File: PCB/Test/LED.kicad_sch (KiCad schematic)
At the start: 45 parts

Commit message: Tidy
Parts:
- TP1, TP2, TP3, TP4, TP5: now left out of the parts list
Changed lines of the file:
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@@
 		(unit 1)
 		(exclude_from_sim no)
-		(in_bom yes)
+		(in_bom no)
 		(on_board yes)
 		(dnp no)
@@
 		(unit 1)
 		(exclude_from_sim no)
-		(in_bom yes)
+		(in_bom no)
 		(on_board yes)
 		(dnp no)
@@
 		(unit 1)
 		(exclude_from_sim no)
-		(in_bom yes)
+		(in_bom no)
 		(on_board yes)
 		(dnp no)
@@
 		(unit 1)
 		(exclude_from_sim no)
-		(in_bom yes)
+		(in_bom no)
 		(on_board yes)
 		(dnp no)
@@
 		(unit 1)
 		(exclude_from_sim no)
-		(in_bom yes)
-		(on_board yes)
-		(dnp no)
+		(in_bom no)
+		(on_board yes)
+		(dnp no)

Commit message: Tweaked design
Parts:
- D11, D12, D13, D14, D15, D16, D17, D18, D19, D20: value XL-1010RGBC-WS2812B -> XL-1615RGBC-WS2812B
- D21, D22, D23, D24, D25, D26, D27, D28, D29, D30, D31, D32, D33, D34, D35, D36, D37, D38, D39, D40: value XL-1010RGBC-WS2812B -> XL-2020RGBC-WS2812B
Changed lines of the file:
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@@
 			)
 		)
-		(property "Value" "XL-1010RGBC-WS2812B"
+		(property "Value" "XL-1615RGBC-WS2812B"
 			(at 160.02 99.06 0)
 			(effects
@@
 			)
 		)
-		(property "Value" "XL-1010RGBC-WS2812B"
+		(property "Value" "XL-2020RGBC-WS2812B"
 			(at 113.665 139.065 0)
 			(effects
@@
 			)
 		)
-		(property "Value" "XL-1010RGBC-WS2812B"
+		(property "Value" "XL-1615RGBC-WS2812B"
 			(at 137.16 99.06 0)
 			(effects
@@
 			)
 		)
-		(property "Value" "XL-1010RGBC-WS2812B"
+		(property "Value" "XL-2020RGBC-WS2812B"
 			(at 174.625 139.065 0)
 			(effects
@@
 			)
 		)
-		(property "Value" "XL-1010RGBC-WS2812B"
+		(property "Value" "XL-1615RGBC-WS2812B"
 			(at 144.78 99.06 0)
 			(effects
@@
 			)
 		)
-		(property "Value" "XL-1010RGBC-WS2812B"
+		(property "Value" "XL-2020RGBC-WS2812B"
 			(at 113.665 119.38 0)
 			(effects
@@
 			)
 		)
-		(property "Value" "XL-1010RGBC-WS2812B"
+		(property "Value" "XL-1615RGBC-WS2812B"
 			(at 121.92 99.06 0)
 			(effects
@@
 			)
 		)
-		(property "Value" "XL-1010RGBC-WS2812B"
+		(property "Value" "XL-1615RGBC-WS2812B"
 			(at 175.26 99.06 0)
 			(effects
@@
 			)
 		)
-		(property "Value" "XL-1010RGBC-WS2812B"
+		(property "Value" "XL-2020RGBC-WS2812B"
 			(at 159.385 119.38 0)
 			(effects
@@
 			)
 		)
-		(property "Value" "XL-1010RGBC-WS2812B"
+		(property "Value" "XL-2020RGBC-WS2812B"
 			(at 144.145 139.065 0)
 			(effects
@@
 			)
 		)
-		(property "Value" "XL-1010RGBC-WS2812B"
+		(property "Value" "XL-2020RGBC-WS2812B"
 			(at 106.045 139.065 0)
 			(effects
@@
 			)
 		)
-		(property "Value" "XL-1010RGBC-WS2812B"
+		(property "Value" "XL-2020RGBC-WS2812B"
 			(at 144.145 119.38 0)
 			(effects
@@
 			)
 		)
-		(property "Value" "XL-1010RGBC-WS2812B"
+		(property "Value" "XL-2020RGBC-WS2812B"
 			(at 106.045 119.38 0)
 			(effects
@@
 			)
 		)
-		(property "Value" "XL-1010RGBC-WS2812B"
+		(property "Value" "XL-2020RGBC-WS2812B"
 			(at 136.525 139.065 0)
 			(effects
@@
 			)
 		)
-		(property "Value" "XL-1010RGBC-WS2812B"
+		(property "Value" "XL-2020RGBC-WS2812B"
 			(at 151.765 119.38 0)
 			(effects
@@
 			)
 		)
-		(property "Value" "XL-1010RGBC-WS2812B"
+		(property "Value" "XL-1615RGBC-WS2812B"
 			(at 152.4 99.06 0)
 			(effects
@@
 			)
 		)
-		(property "Value" "XL-1010RGBC-WS2812B"
+		(property "Value" "XL-2020RGBC-WS2812B"
 			(at 121.285 119.38 0)
 			(effects
@@
 			)
 		)
-		(property "Value" "XL-1010RGBC-WS2812B"
+		(property "Value" "XL-2020RGBC-WS2812B"
 			(at 174.625 119.38 0)
 			(effects
@@
 			)
 		)
-		(property "Value" "XL-1010RGBC-WS2812B"
+		(property "Value" "XL-2020RGBC-WS2812B"
 			(at 159.385 139.065 0)
 			(effects
@@
 			)
 		)
-		(property "Value" "XL-1010RGBC-WS2812B"
+		(property "Value" "XL-1615RGBC-WS2812B"
 			(at 129.54 99.06 0)
 			(effects
@@
 			)
 		)
-		(property "Value" "XL-1010RGBC-WS2812B"
+		(property "Value" "XL-1615RGBC-WS2812B"
 			(at 167.64 99.06 0)
 			(effects
@@
 			)
 		)
-		(property "Value" "XL-1010RGBC-WS2812B"
+		(property "Value" "XL-2020RGBC-WS2812B"
 			(at 167.005 119.38 0)
 			(effects
@@
 			)
 		)
-		(property "Value" "XL-1010RGBC-WS2812B"
+		(property "Value" "XL-2020RGBC-WS2812B"
 			(at 121.285 139.065 0)
 			(effects
@@
 			)
 		)
-		(property "Value" "XL-1010RGBC-WS2812B"
+		(property "Value" "XL-2020RGBC-WS2812B"
 			(at 167.005 139.065 0)
 			(effects
@@
 			)
 		)
-		(property "Value" "XL-1010RGBC-WS2812B"
+		(property "Value" "XL-2020RGBC-WS2812B"
 			(at 128.905 119.38 0)
 			(effects
@@
 			)
 		)
-		(property "Value" "XL-1010RGBC-WS2812B"
+		(property "Value" "XL-2020RGBC-WS2812B"
 			(at 151.765 139.065 0)
 			(effects
@@
 			)
 		)
-		(property "Value" "XL-1010RGBC-WS2812B"
+		(property "Value" "XL-2020RGBC-WS2812B"
 			(at 128.905 139.065 0)
 			(effects
@@
 			)
 		)
-		(property "Value" "XL-1010RGBC-WS2812B"
+		(property "Value" "XL-2020RGBC-WS2812B"
 			(at 136.525 119.38 0)
 			(effects
@@
 			)
 		)
-		(property "Value" "XL-1010RGBC-WS2812B"
+		(property "Value" "XL-1615RGBC-WS2812B"
 			(at 106.68 99.06 0)
 			(effects
@@
 			)
 		)
-		(property "Value" "XL-1010RGBC-WS2812B"
+		(property "Value" "XL-1615RGBC-WS2812B"
 			(at 114.3 99.06 0)
 			(effects

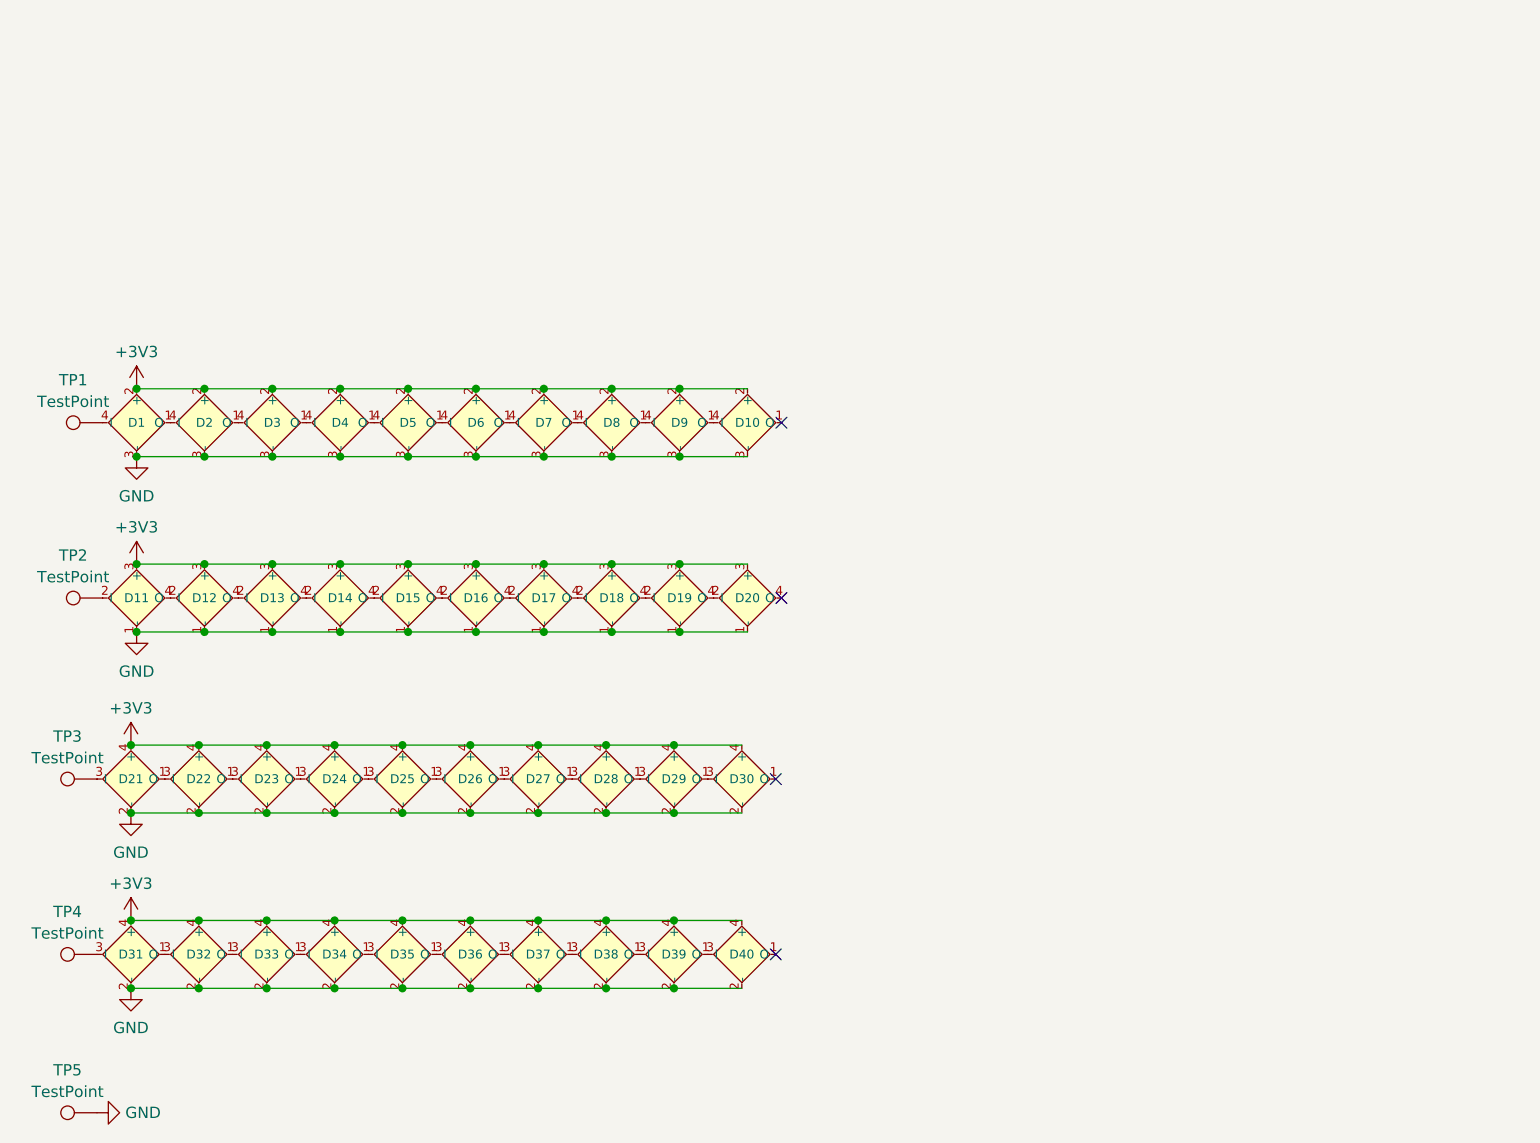
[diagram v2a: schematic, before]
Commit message: Update test seven seg
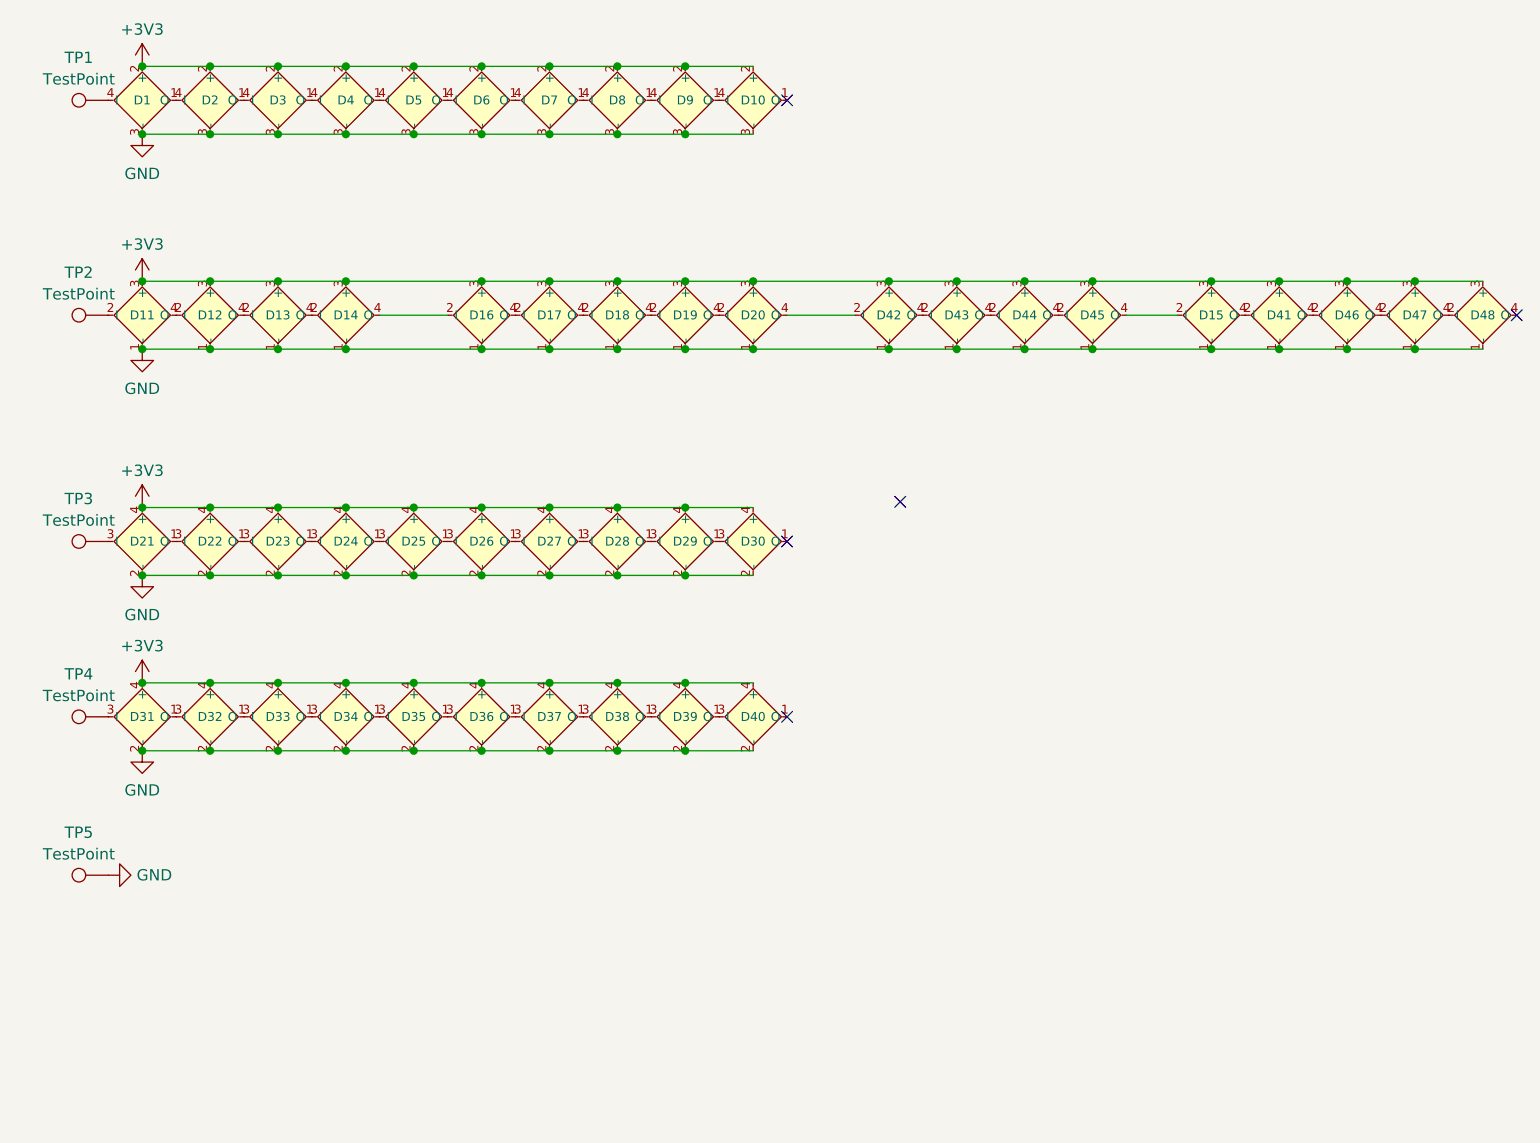
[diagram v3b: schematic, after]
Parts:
- added D41, D42, D43, D44, D45, D46, D47, D48: XL-1615RGBC-WS2812B, RevK:SMD1615, symbol RevK:WS2812B-1.5mm
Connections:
- net +3V3: now also D41.3 (+), D42.3 (+), D43.3 (+), D44.3 (+), D45.3 (+), D46.3 (+), D47.3 (+), D48.3 (+)
- net GND: now also D41.1 (-), D42.1 (-), D43.1 (-), D44.1 (-), D45.1 (-), D46.1 (-), D47.1 (-), D48.1 (-)
- net at D14.4 (O): now also D16.2 (I); no longer D15.2 (I)
- net at D15.4 (O): now also D41.2 (I); no longer D16.2 (I)
- net at D20.4 (O): now also D42.2 (I)
- new net: D47.4 (O), D48.2 (I)
- new net: D44.4 (O), D45.2 (I)
- new net: D15.2 (I), D45.4 (O)
- new net: D41.4 (O), D46.2 (I)
- new net: D46.4 (O), D47.2 (I)
- new net: D43.4 (O), D44.2 (I)
- new net: D42.4 (O), D43.2 (I)
- no-connect marks 4 -> 5
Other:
- moved on the sheet: D1, D10, D11, D12, D13, D14, D16, D17, D18, D19, D2, D20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
